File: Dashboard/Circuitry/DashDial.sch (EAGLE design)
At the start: 33 parts, among them IC1 TLC5947DAPR, U1 LOGIC SHIFTER, X2 SERVO, X3 POWER, X4 LOGIC

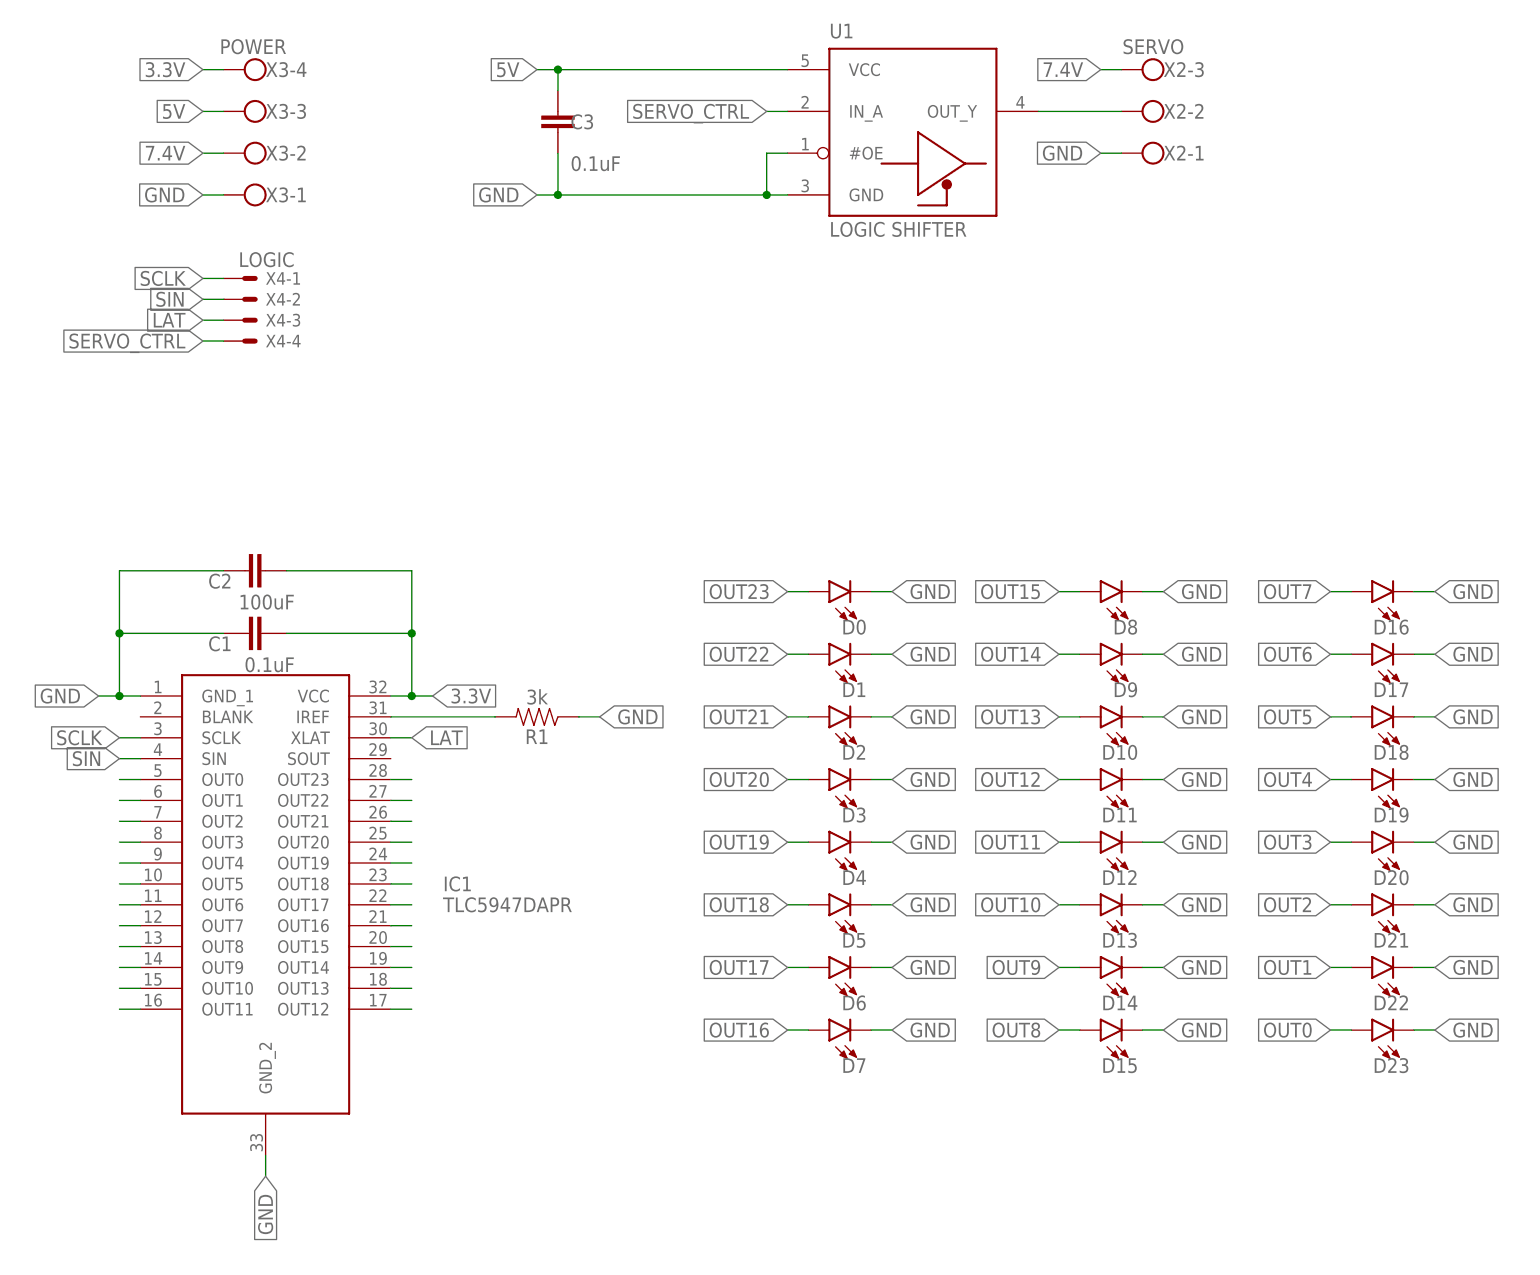
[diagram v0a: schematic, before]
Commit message: Finished redesign of DashDial
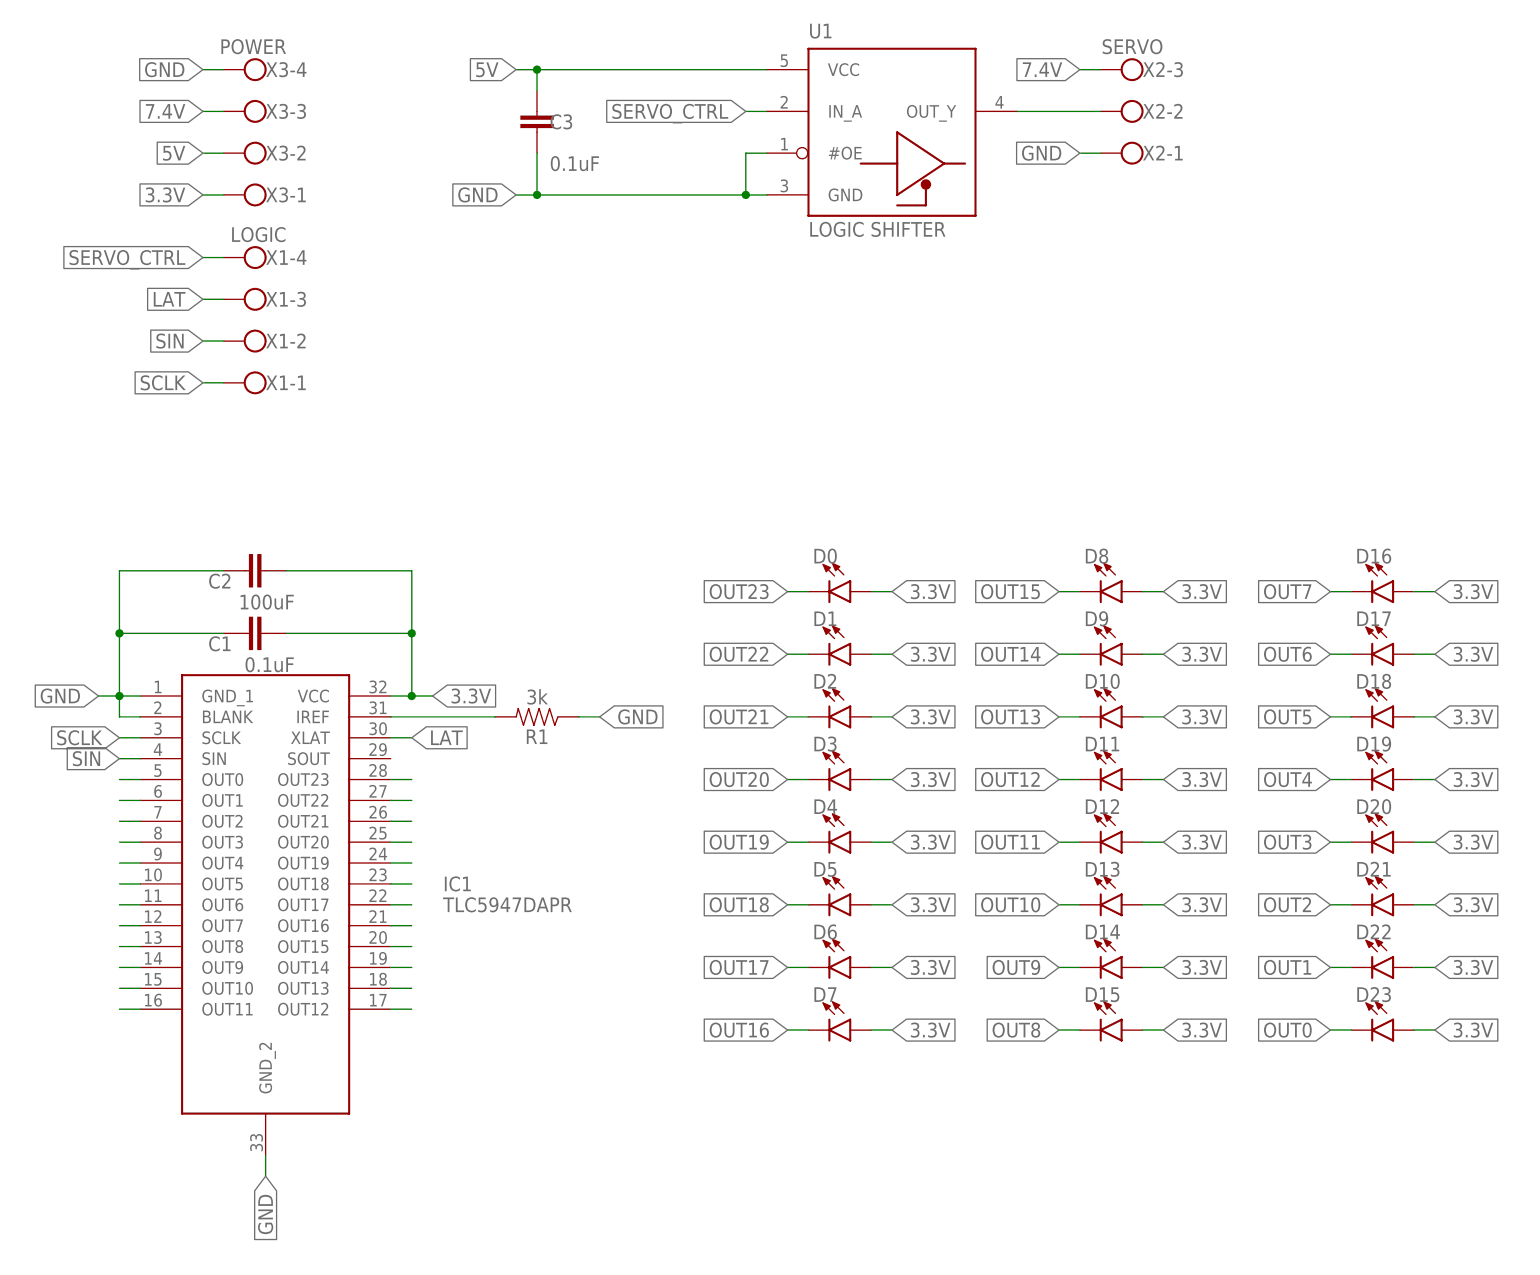
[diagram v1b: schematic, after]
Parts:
- removed X4: LOGIC, Rembrandt Electronics - JST XH Connectors v1-0:JST-XH-04-PIN-LONG-PAD
- added X1: LOGIC, con-wago-500:W237-4
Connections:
- net 3.3V: now also D0.A, D1.A, D10.A, D11.A, D12.A, D13.A, D14.A, D15.A, D16.A, D17.A, D18.A, D19.A, D2.A, D20.A, D21.A, D22.A, D23.A, D3.A, D4.A, D5.A, D6.A, D7.A, D8.A, D9.A, X3-1.KL; no longer X3-4.KL
- net 5V: now also X3-2.KL; no longer X3-3.KL
- net 7.4V: now also X3-3.KL; no longer X3-2.KL
- net GND: now also IC1.BLANK, X3-4.KL; no longer D0.C, D1.C, D10.C, D11.C, D12.C, D13.C, D14.C, D15.C, D16.C, D17.C, D18.C, D19.C, D2.C, D20.C, D21.C, D22.C, D23.C, D3.C, D4.C, D5.C, D6.C, D7.C, D8.C, D9.C, X3-1.KL
- net LAT: now also X1-3.KL; no longer X4-3.S
- net OUT0: now also D23.C; no longer D23.A
- net OUT1: now also D22.C; no longer D22.A
- net OUT10: now also D13.C; no longer D13.A
- net OUT11: now also D12.C; no longer D12.A
- net OUT12: now also D11.C; no longer D11.A
- net OUT13: now also D10.C; no longer D10.A
- net OUT14: now also D9.C; no longer D9.A
- net OUT15: now also D8.C; no longer D8.A
- net OUT16: now also D7.C; no longer D7.A
- net OUT17: now also D6.C; no longer D6.A
- net OUT18: now also D5.C; no longer D5.A
- net OUT19: now also D4.C; no longer D4.A
- net OUT2: now also D21.C; no longer D21.A
- net OUT20: now also D3.C; no longer D3.A
- net OUT21: now also D2.C; no longer D2.A
- net OUT22: now also D1.C; no longer D1.A
- net OUT23: now also D0.C; no longer D0.A
- net OUT3: now also D20.C; no longer D20.A
- net OUT4: now also D19.C; no longer D19.A
- net OUT5: now also D18.C; no longer D18.A
- net OUT6: now also D17.C; no longer D17.A
- net OUT7: now also D16.C; no longer D16.A
- net OUT8: now also D15.C; no longer D15.A
- net OUT9: now also D14.C; no longer D14.A
- net SCLK: now also X1-1.KL; no longer X4-1.S
- net SERVO_CTRL: now also X1-4.KL; no longer X4-4.S
- net SIN: now also X1-2.KL; no longer X4-2.S
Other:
- note added: "DashDial V2 Designer: Akash Harapanahalli"
- note removed: "DashDial V1 Designer: Akash Harapanahalli"
- moved on the sheet: C3, D0, D1, D10, D11, D12, D13, D14, D15, D16, D17, D18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
